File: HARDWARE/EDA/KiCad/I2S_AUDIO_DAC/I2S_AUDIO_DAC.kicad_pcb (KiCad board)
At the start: 2 copper layers, 32 parts, among them J1 Conn_01x07_Male, J2 Conn_01x010_Male, U1 L78L33_TO92, U2 UDA1334ATS

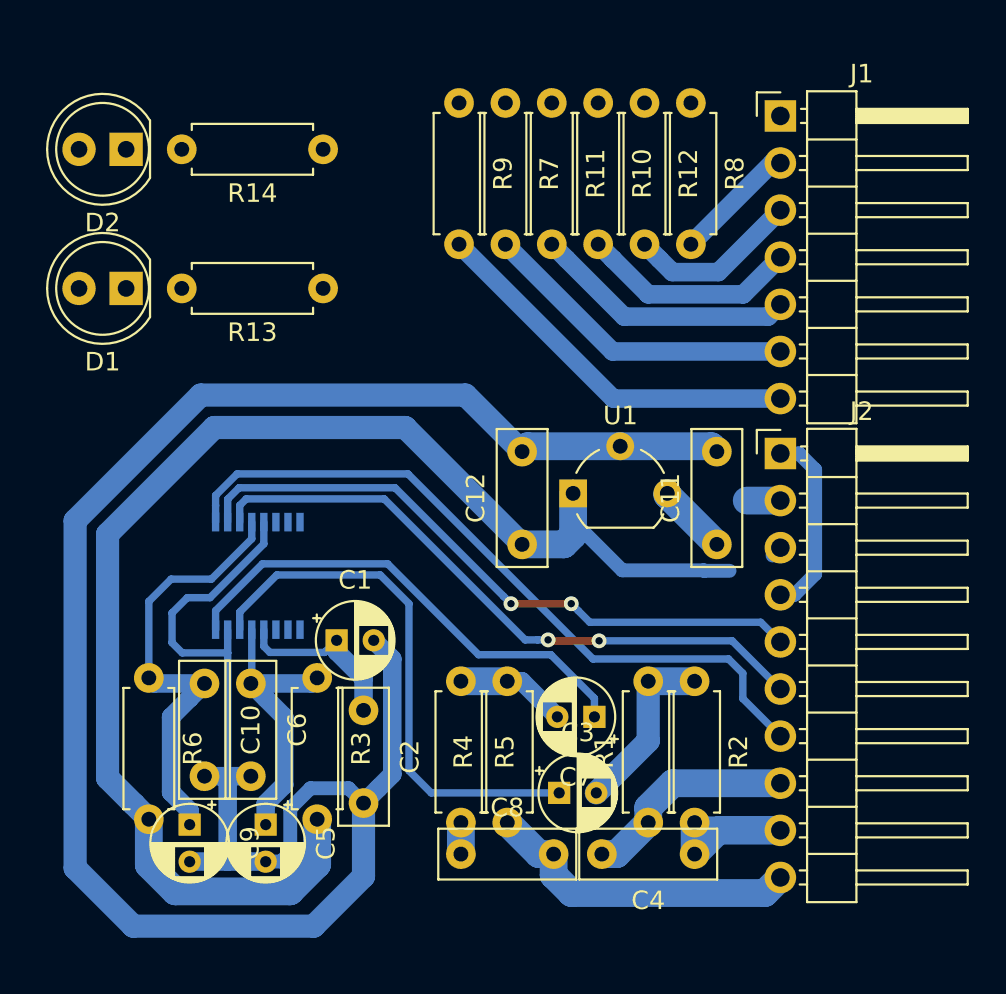
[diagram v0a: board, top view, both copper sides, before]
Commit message: pcb finished
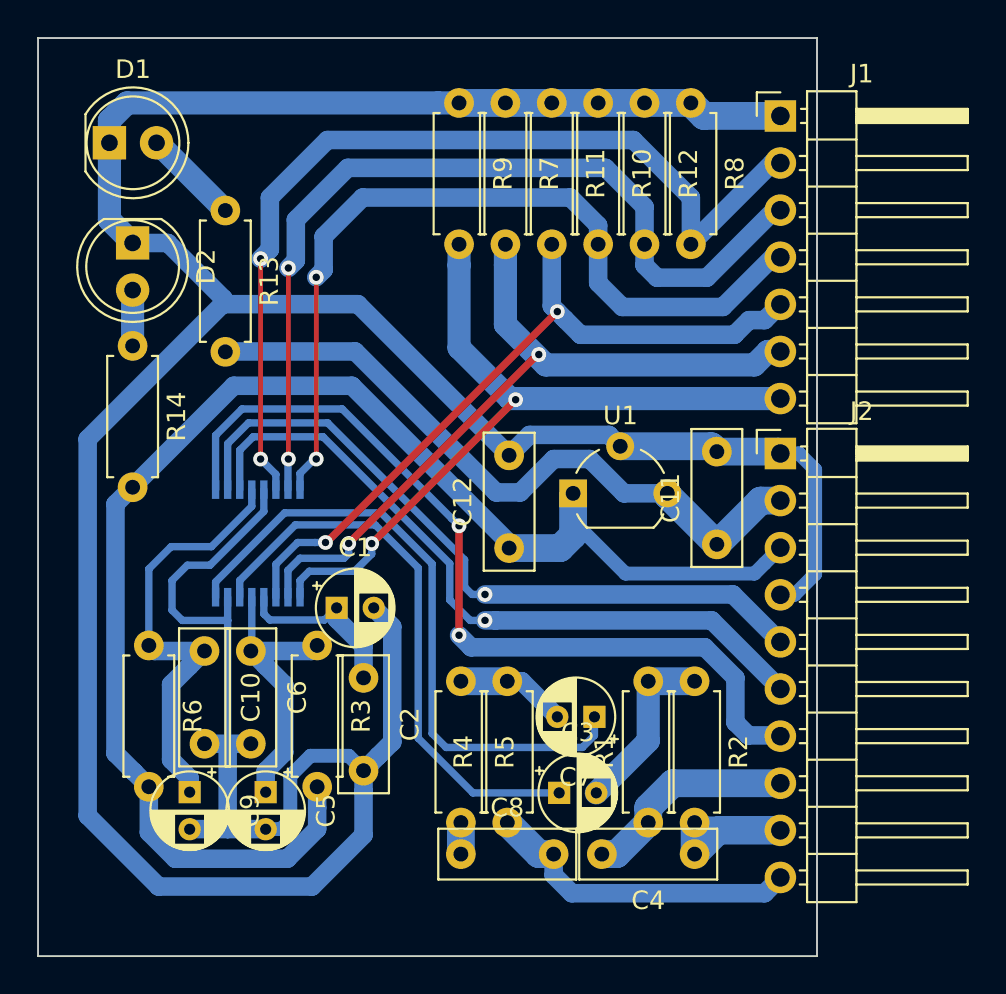
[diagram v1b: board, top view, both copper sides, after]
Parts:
- moved R14 14.8 mm to (179.1, 87.1), turned to 270 degrees
- moved D1 7.90 mm to (177.8, 76.2), turned to 0 degrees
- moved R13 6.74 mm to (184.1, 79.8), turned to 270 degrees
- moved D2 5.06 mm to (179.1, 81.5), turned to 270 degrees
- moved C1 1.75 mm to (190.1, 101.2)
- moved C10 1.75 mm to (183.0, 103.5)
- moved C2 1.75 mm to (191.5, 105.0)
- moved C5 1.75 mm to (186.3, 111.2)
- moved C6 1.75 mm to (185.5, 103.6)
- moved C9 1.75 mm to (182.2, 111.2)
- moved R3 1.75 mm to (189.0, 103.2)
- moved R6 1.75 mm to (180.0, 103.3)
- moved U2 1.75 mm to (185.8, 97.8)
- moved C12 0.73 mm to (199.4, 98.0)
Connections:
- D1 pad 1: Net-(D1-Pad1) -> 0
- D1 pad 2: VDC -> Net-(D1-Pad2)
- D2 pad 1: Net-(D2-Pad1) -> 0
- D2 pad 2: analog_supply_voltage -> Net-(D2-Pad2)
- R13 pad 1: 0 -> Net-(D1-Pad2)
- R13 pad 2: Net-(D1-Pad1) -> VDC
- R14 pad 1: 0 -> Net-(D2-Pad2)
- R14 pad 2: Net-(D2-Pad1) -> analog_supply_voltage
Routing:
- net 0: track 139.8 -> 196.7 mm
- net /SYSCLK_IN: track 6.64 -> 50.7 mm, vias 0 -> 2
- net /SFOR1: track 9.33 -> 47.8 mm, vias 0 -> 2
- net /MUTE: track 11.8 -> 45.2 mm, vias 0 -> 2
- net VDC: track 5.67 -> 36.8 mm
- net /SFOR0: track 14.2 -> 39.6 mm, vias 0 -> 2
- net /PLL_IN: track 17.2 -> 40.5 mm, vias 0 -> 2
- net /DEEM-CLKOUT: track 20.8 -> 40.9 mm, vias 0 -> 2
- net VOUTR: track 26.5 -> 34.7 mm
- net /BITCLK_IN: track 39.0 -> 46.1 mm, vias 0 -> 2
- net Net-(D1-Pad2): track 0.00 -> 5.22 mm
- net /DATA_IN: track 34.4 -> 38.4 mm, vias 2 -> 1
- net /WORDSEL_IN: track 34.7 -> 38.5 mm, vias 2 -> 1
- net analog_supply_voltage: track 75.6 -> 79.1 mm
- net Net-(D2-Pad2): track 0.00 -> 2.98 mm
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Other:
- board outline added: 42 x 49.5 mm
- net class Default: clearance 0.5 -> 0.25
- rule trace_clearance: 0.5 -> 0.25
